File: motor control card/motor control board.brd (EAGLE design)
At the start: 100 x 80 mm, 13 parts, among them J1 09231486921, J2 TBP02R1-381-07BE, J3 TBP02R1-381-07BE

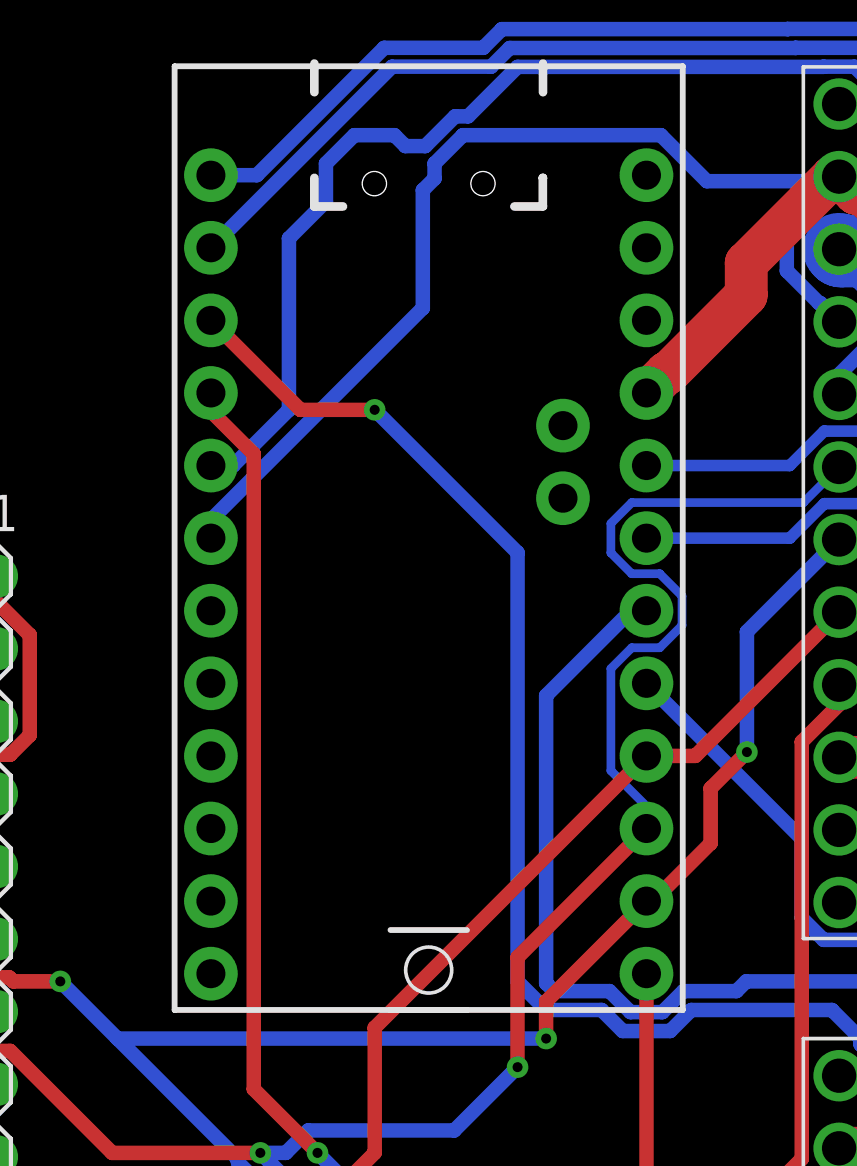
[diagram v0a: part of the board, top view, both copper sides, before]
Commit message: added cam data
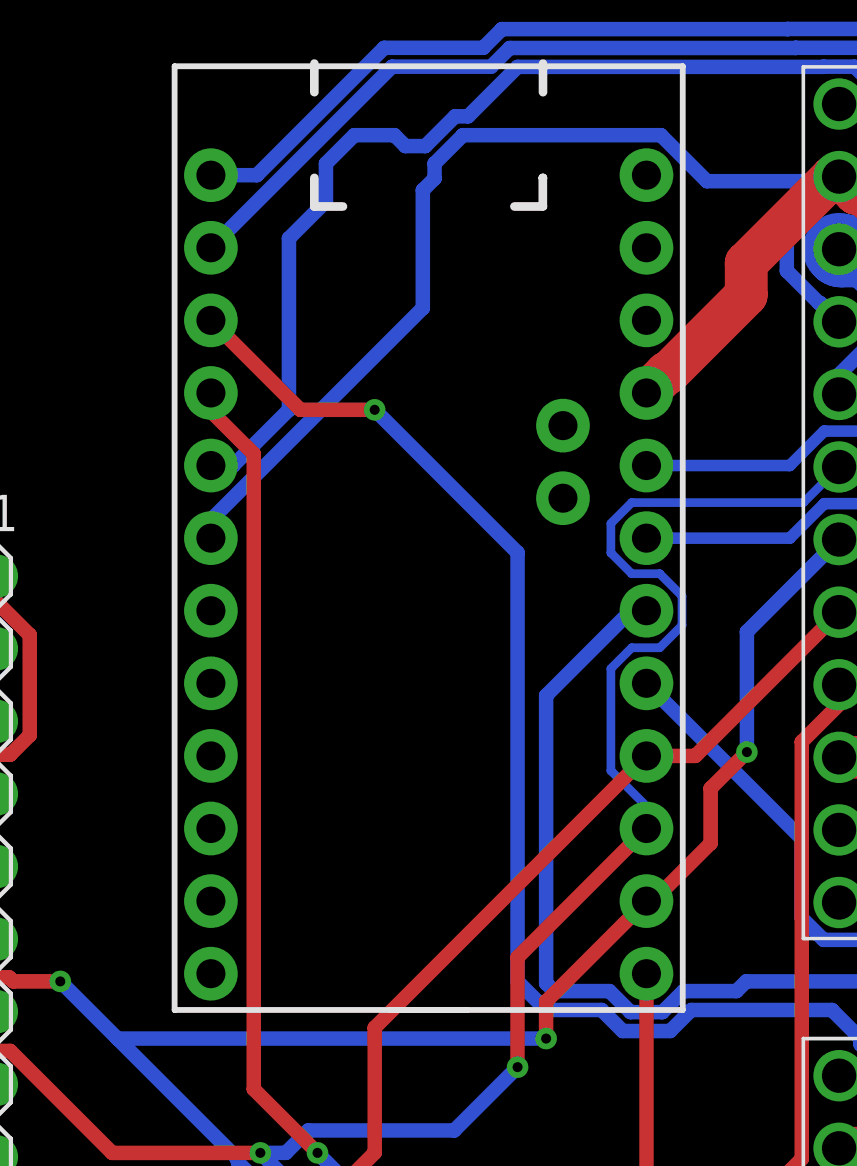
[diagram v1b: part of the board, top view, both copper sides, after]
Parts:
- U$1, U$2: device high power stepper driver 36V4:BREAKOUT_BOARD -> high_power_stepper_driver_36V4:BREAKOUT_BOARD
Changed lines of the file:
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@@
 <attribute name="VALUE" x="-8.59" y="67.73" locked="yes" size="1.27" layer="27" rot="R270"/>
 </element>
-<element name="U$1" library="high power stepper driver 36V4" package="BREAKOUT_BOARD" value="POLOLU_HIGH-POWER_STEPPER_MOTOR_DRIVER_36V4" x="84" y="75" locked="yes" smashed="yes" rot="R180"/>
-<element name="U$3" library="SparkFun-SAMD21-Mini-Breakout" package="JP1_SPARKFUN-SAMD21-MINI-BREAKOUT-V10" value="" x="29" y="42" locked="yes" smashed="yes"/>
-<element name="U$2" library="high power stepper driver 36V4" package="BREAKOUT_BOARD" value="POLOLU_HIGH-POWER_STEPPER_MOTOR_DRIVER_36V4" x="84" y="41" smashed="yes" rot="R180"/>
+<element name="U$1" library="high_power_stepper_driver_36V4" package="BREAKOUT_BOARD" value="POLOLU_HIGH-POWER_STEPPER_MOTOR_DRIVER_36V4" x="84" y="75" locked="yes" smashed="yes" rot="R180">
+<attribute name="PURCHASE_URL_POLOLU" value="https://www.pololu.com/product/3730/resources" x="84" y="75" size="1.778" layer="27" rot="R180" display="off"/>
+</element>
+<element name="U$3" library="SparkFun-SAMD21-Mini-Breakout" package="JP1_SPARKFUN-SAMD21-MINI-BREAKOUT-V10" value="" x="29" y="42" locked="yes" smashed="yes">
+<attribute name="PURCHASE_URL_DIGIKEY" value="https://www.digikey.ca/en/products/detail/sparkfun-electronics/DEV-13664/5766914?s=N4IgTCBcDaIM4EMC2ATMBGABEglgOx0wCMAnAUwQGsB7AVwBcQBdAXyA" x="29" y="42" size="1.778" layer="27" display="off"/>
+<attribute name="PURCHASE_URL_SPARKFUN" value="https://www.sparkfun.com/products/13664" x="29" y="42" size="1.778" layer="27" display="off"/>
+</element>
+<element name="U$2" library="high_power_stepper_driver_36V4" package="BREAKOUT_BOARD" value="POLOLU_HIGH-POWER_STEPPER_MOTOR_DRIVER_36V4" x="84" y="41" smashed="yes" rot="R180">
+<attribute name="PURCHASE_URL_POLOLU" value="https://www.pololu.com/product/3730/resources" x="84" y="41" size="1.778" layer="27" rot="R180" display="off"/>
+</element>
 <element name="J2" library="TBP02R1-381-07BE" package="CUI_TBP02R1-381-07BE" value="TBP02R1-381-07BE" x="91" y="35" locked="yes" smashed="yes" rot="R270">
 <attribute name="AVAILABILITY" value="In Stock" x="91" y="36" locked="yes" size="1.778" layer="27" rot="R270" display="off"/>
@@
 <contactref element="J1" pad="19"/>
 <contactref element="J1" pad="18"/>
-<contactref element="U$3" pad="4@JP1"/>
 <contactref element="J2" pad="3"/>
 <contactref element="J3" pad="3"/>
@@
 <via x="41.5" y="14.8" extent="1-16" drill="0.35"/>
 <via x="42.6" y="14.8" extent="1-16" drill="0.35"/>
-<wire x1="82.73" y1="58.49" x2="91" y2="59.24" width="0" layer="19" extent="1-1"/>
-<wire x1="82.73" y1="55.95" x2="82.73" y2="58.49" width="0" layer="19" extent="1-1"/>
-<wire x1="58" y1="67" x2="82.73" y2="58.49" width="0" layer="19" extent="1-1"/>
-<wire x1="57.1" y1="66.4" x2="58" y2="67" width="0" layer="19" extent="1-1"/>
-<wire x1="57.1" y1="67.7" x2="58" y2="67" width="0" layer="19" extent="1-1"/>
-<wire x1="30.27" y1="50.89" x2="52.25" y2="68.62" width="0" layer="19" extent="1-1"/>
-<wire x1="52.25" y1="34.62" x2="30.27" y2="50.89" width="0" layer="19" extent="1-1"/>
-<wire x1="41" y1="19" x2="52.25" y2="34.62" width="0" layer="19" extent="1-1"/>
-<wire x1="40" y1="19" x2="41" y2="19" width="0" layer="19" extent="1-1"/>
-<wire x1="39.5" y1="18.3" x2="40" y2="19" width="0" layer="19" extent="1-1"/>
-<wire x1="41.5" y1="14.8" x2="42" y2="14" width="0" layer="19" extent="1-1"/>
-<wire x1="42.6" y1="14.8" x2="42" y2="14" width="0" layer="19" extent="1-1"/>
-<wire x1="10.68" y1="21" x2="39.5" y2="18.3" width="0" layer="19" extent="1-1"/>
-<wire x1="10.68" y1="23.54" x2="10.68" y2="21" width="0" layer="19" extent="1-1"/>
-<wire x1="10.68" y1="26.08" x2="10.68" y2="23.54" width="0" layer="19" extent="1-1"/>
-<wire x1="8.14" y1="26.08" x2="10.68" y2="26.08" width="0" layer="19" extent="1-1"/>
-<wire x1="5.6" y1="26.08" x2="8.14" y2="26.08" width="0" layer="19" extent="1-1"/>
-<wire x1="5.6" y1="28.62" x2="5.6" y2="26.08" width="0" layer="19" extent="1-1"/>
-<wire x1="8.14" y1="23.54" x2="10.68" y2="23.54" width="0" layer="19" extent="1-1"/>
-<wire x1="5.6" y1="23.54" x2="5.6" y2="26.08" width="0" layer="19" extent="1-1"/>
-<wire x1="8.14" y1="21" x2="10.68" y2="21" width="0" layer="19" extent="1-1"/>
-<wire x1="5.6" y1="21" x2="5.6" y2="23.54" width="0" layer="19" extent="1-1"/>
-<wire x1="91" y1="27.38" x2="82.73" y2="55.95" width="0" layer="19" extent="1-1"/>
-<wire x1="82.73" y1="24.49" x2="91" y2="27.38" width="0" layer="19" extent="1-1"/>
-<wire x1="82.73" y1="21.95" x2="82.73" y2="24.49" width="0" layer="19" extent="1-1"/>
+<contactref element="U$3" pad="4@JP1"/>
 </signal>
 <signal name="24V/12V">
@@
 <vertex x="5.1" y="33.8"/>
 </polygon>
-<wire x1="82.73" y1="50.87" x2="82.73" y2="53.41" width="0" layer="19" extent="1-1"/>
-<wire x1="82.73" y1="19.41" x2="82.73" y2="50.87" width="0" layer="19" extent="1-1"/>
-<wire x1="82.73" y1="16.87" x2="82.73" y2="19.41" width="0" layer="19" extent="1-1"/>
-<wire x1="10.68" y1="28.62" x2="82.73" y2="19.41" width="0" layer="19" extent="1-1"/>
-<wire x1="10.68" y1="31.16" x2="10.68" y2="28.62" width="0" layer="19" extent="1-1"/>
-<wire x1="8.14" y1="31.16" x2="10.68" y2="31.16" width="0" layer="19" extent="1-1"/>
-<wire x1="8.14" y1="33.7" x2="8.14" y2="31.16" width="0" layer="19" extent="1-1"/>
-<wire x1="5.6" y1="33.7" x2="8.14" y2="33.7" width="0" layer="19" extent="1-1"/>
-<wire x1="5.6" y1="31.16" x2="8.14" y2="31.16" width="0" layer="19" extent="1-1"/>
-<wire x1="8.14" y1="28.62" x2="10.68" y2="28.62" width="0" layer="19" extent="1-1"/>
 </signal>
 <signal name="5V">
@@
 <mfgpreviewcolor name="substratecolor" color="0xFF786E46"/>
 </mfgpreviewcolors>
+<errors>
+</errors>
 </board>
 </drawing>
